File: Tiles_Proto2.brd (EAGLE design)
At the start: 100 x 80 mm, 47 parts, among them J1 7p-SMD-2.54, U1 ADXL345BCCZ-RL, U2 MPR121QR2, U3 MCP73832T-2ACI/OT-SOT23-5

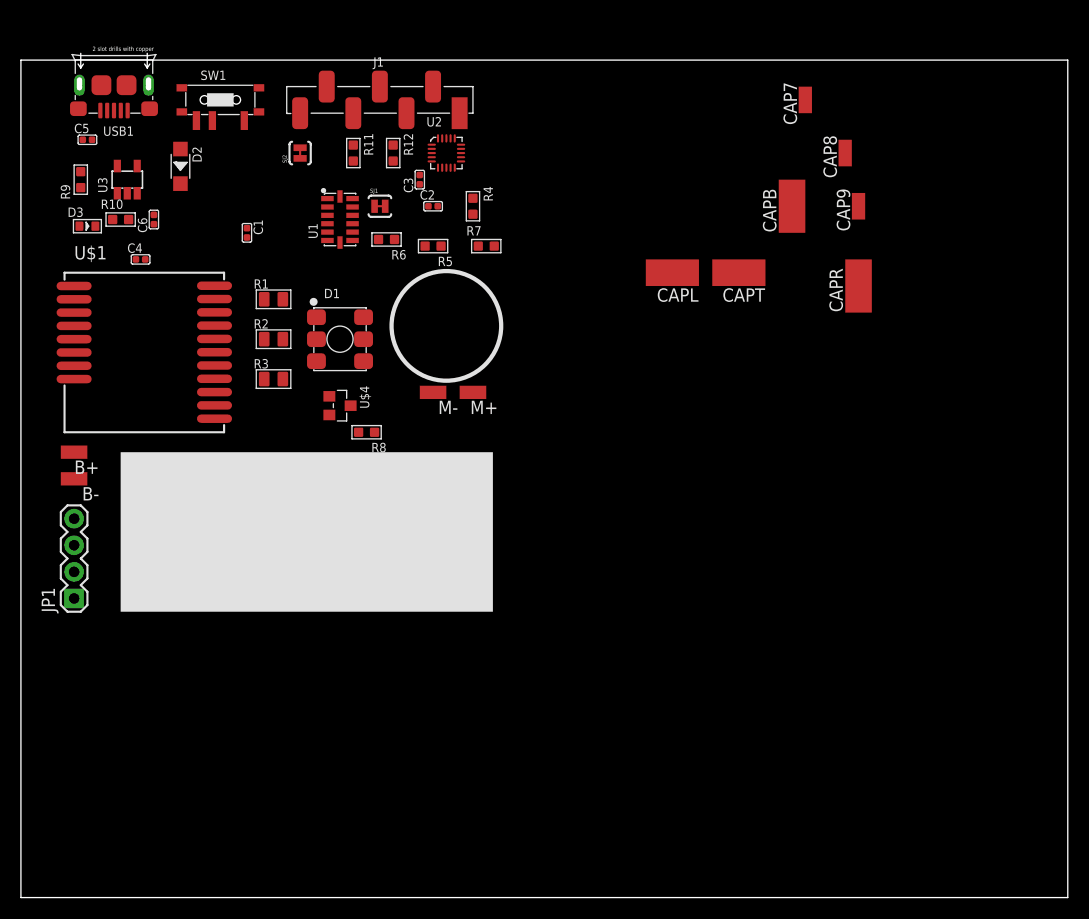
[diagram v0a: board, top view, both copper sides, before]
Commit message: version before starting routing
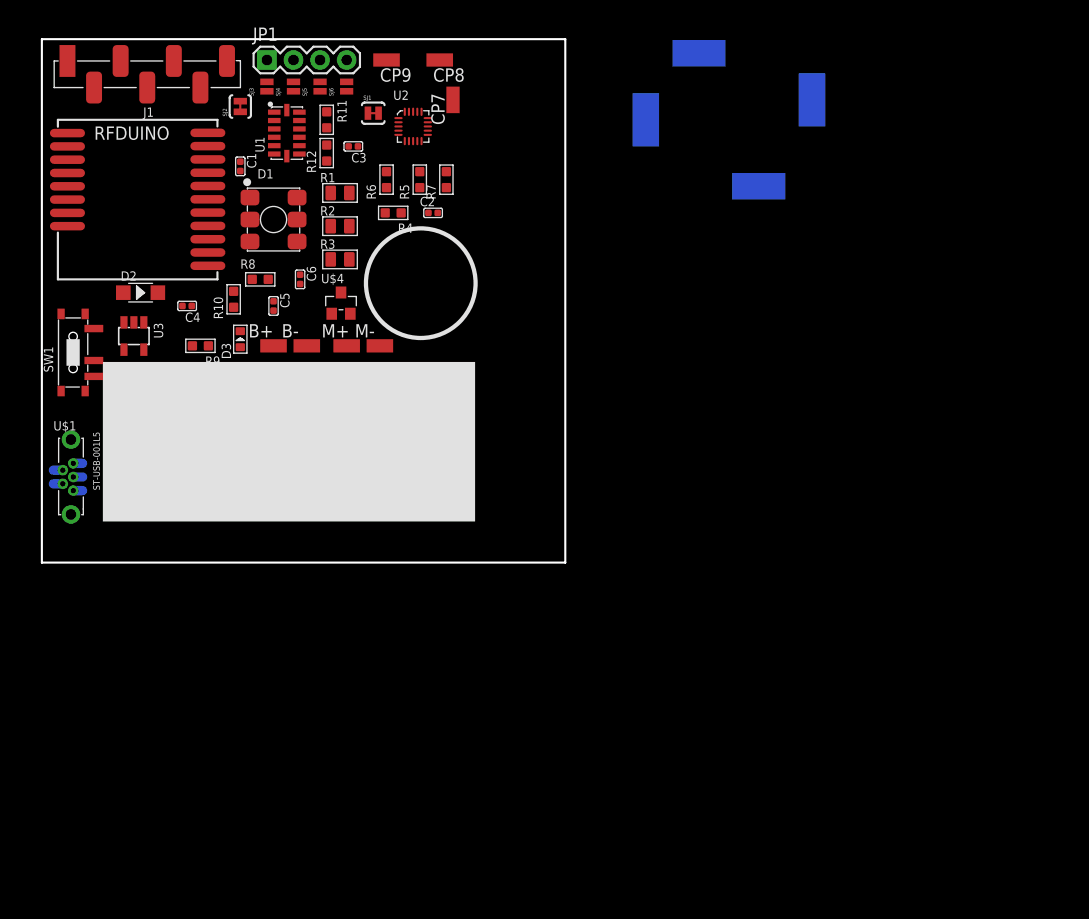
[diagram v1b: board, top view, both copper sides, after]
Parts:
- removed CAP7, CAP8, CAP9: (no value), wirepad:SMD1,27-2,54
- removed USB1: 10118193-0001LF, Seeed-OPL-Connector:MICRO-USB5+6P-SMD-0.65-B
- added CP7, CP8, CP9: (no value), wirepad:SMD1,27-2,54
- added RFDUINO: RF22301, GeekAmmo:RFD22301
- U$1: value RF22301 -> ST-USB-001L5; device GeekAmmo:RFD22301 -> Seeed-OPL-Connector:MICRO-USB5+2P-0.65-180D
- moved JP1 54.6 mm to (23.5, 80.0), turned to 0 degrees
- moved SJ3 45.8 mm to (23.5, 77.5)
- moved SJ4 45.8 mm to (26.0, 77.5)
- moved SJ5 45.8 mm to (28.6, 77.5)
- moved SJ6 45.8 mm to (31.1, 77.5)
- moved SW1 27.9 mm to (4.99, 52.1), turned to 0 degrees
- moved B- 25.6 mm to (27.3, 52.7), turned to 270 degrees
- moved C5 23.8 mm to (24.1, 56.5), turned to 0 degrees
- moved J1 22.4 mm to (12.1, 78.6), turned to 90 degrees
- moved B+ 21.6 mm to (24.1, 52.7), turned to 270 degrees
- moved CAPL 21.1 mm to (64.8, 80.6), flipped to the bottom
- moved R9 19.6 mm to (17.1, 52.7), turned to 90 degrees
- moved CAPR 18.3 mm to (75.6, 76.2), flipped to the bottom
- moved U$1 18.2 mm to (5.00, 40.2)
- moved D3 18.2 mm to (21.0, 53.3), turned to 90 degrees
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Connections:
- net FACTORY: now also RFDUINO.15; no longer U$1.15
- net GND: now also R1.2, R2.2, R3.2, RFDUINO.1, RFDUINO.10, RFDUINO.12, RFDUINO.18, RFDUINO.19, RFDUINO.2, RFDUINO.8, RFDUINO.9, U$1.5; no longer D1.4, D1.5, D1.6, U$1.1, U$1.10, U$1.12, U$1.18, U$1.19, U$1.2, U$1.8, U$1.9, USB1.5
- net HAPTIC: now also RFDUINO.4; no longer U$1.4
- net INT: now also RFDUINO.5; no longer U$1.5
- net LED_B: now also D1.3, RFDUINO.3; no longer R3.1, U$1.3
- net LED_G: now also D1.2, RFDUINO.17; no longer R1.1, U$1.17
- net LED_R: now also D1.1, RFDUINO.16; no longer R2.1, U$1.16
- net N$1: now also D1.5, R1.1; no longer D1.2, R1.2
- net N$2: now also D1.6, R2.1; no longer D1.1, R2.2
- net N$20: now also CP7.1; no longer CAP7.1
- net N$21: now also CP8.1; no longer CAP8.1
- net N$22: now also CP9.1; no longer CAP9.1
- net N$3: now also D1.4, R3.1; no longer D1.3, R3.2
- net N$8: now also U$1.1; no longer USB1.1
- net RESET: now also RFDUINO.14; no longer U$1.14
- net SCL: now also RFDUINO.6; no longer U$1.6
- net SDA: now also RFDUINO.7; no longer U$1.7
- net VCC: now also RFDUINO.13; no longer U$1.13
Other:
- board size 100 x 80 mm -> 50 x 50 mm
